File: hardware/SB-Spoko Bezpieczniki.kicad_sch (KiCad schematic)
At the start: 20 parts, among them IC1 STM32L4P5RET6, SW1 RESET, Y1 Crystal_GND24_Small

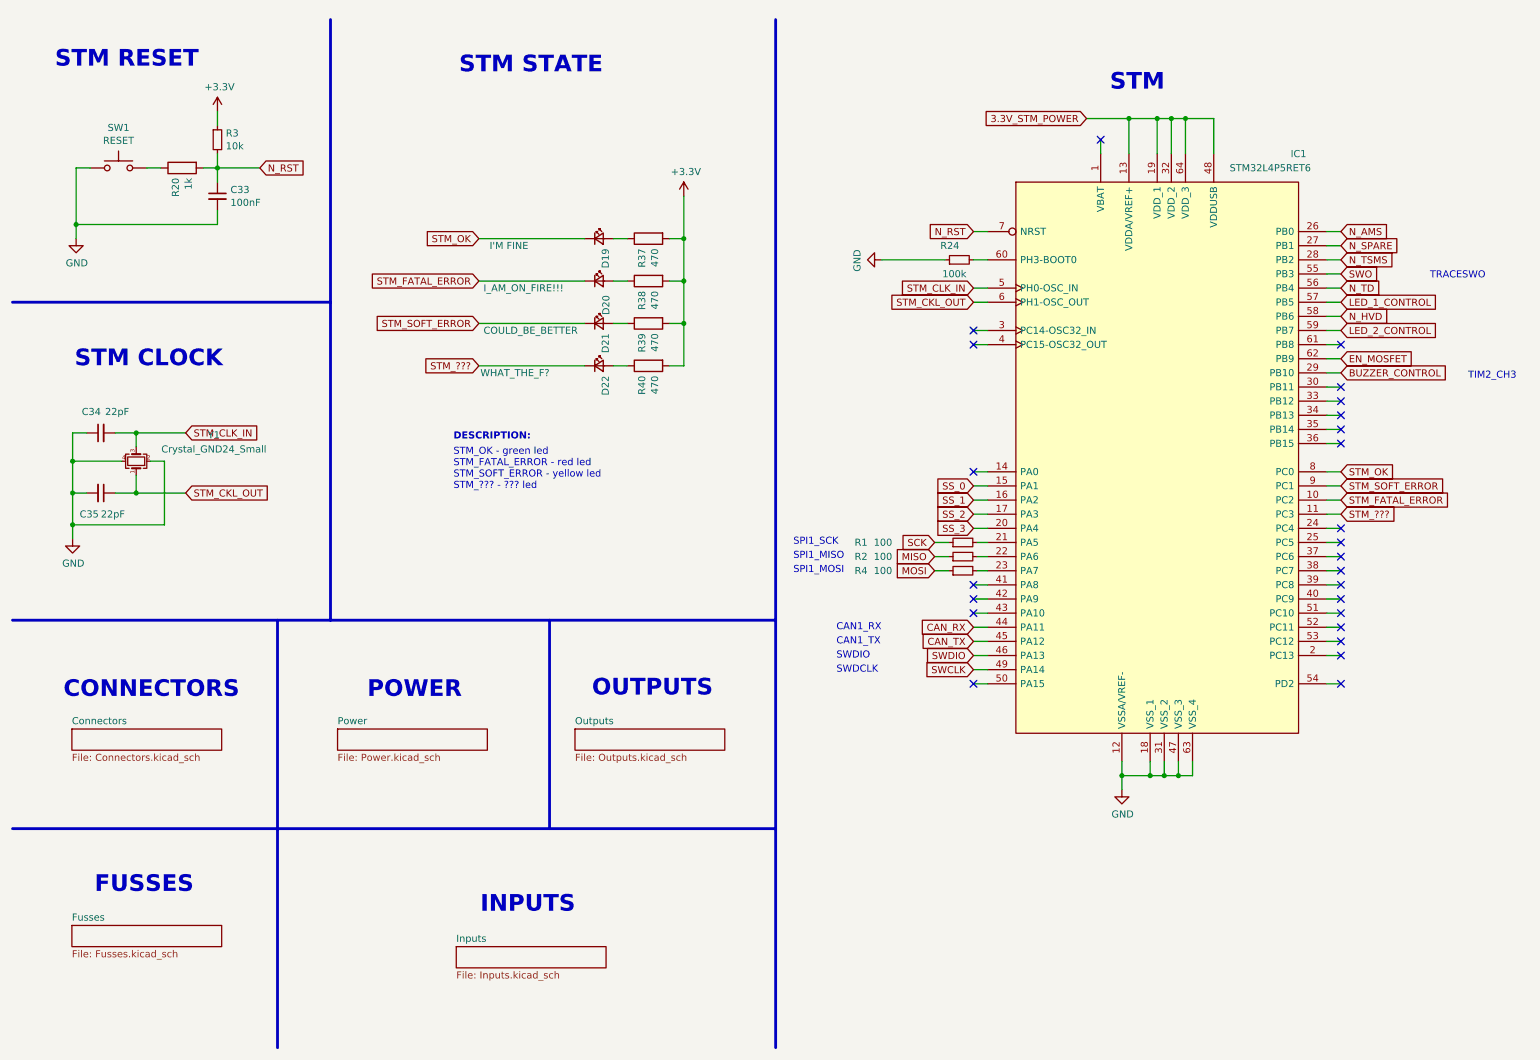
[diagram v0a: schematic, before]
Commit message: changed some footprints for clarity, and made some progress on board
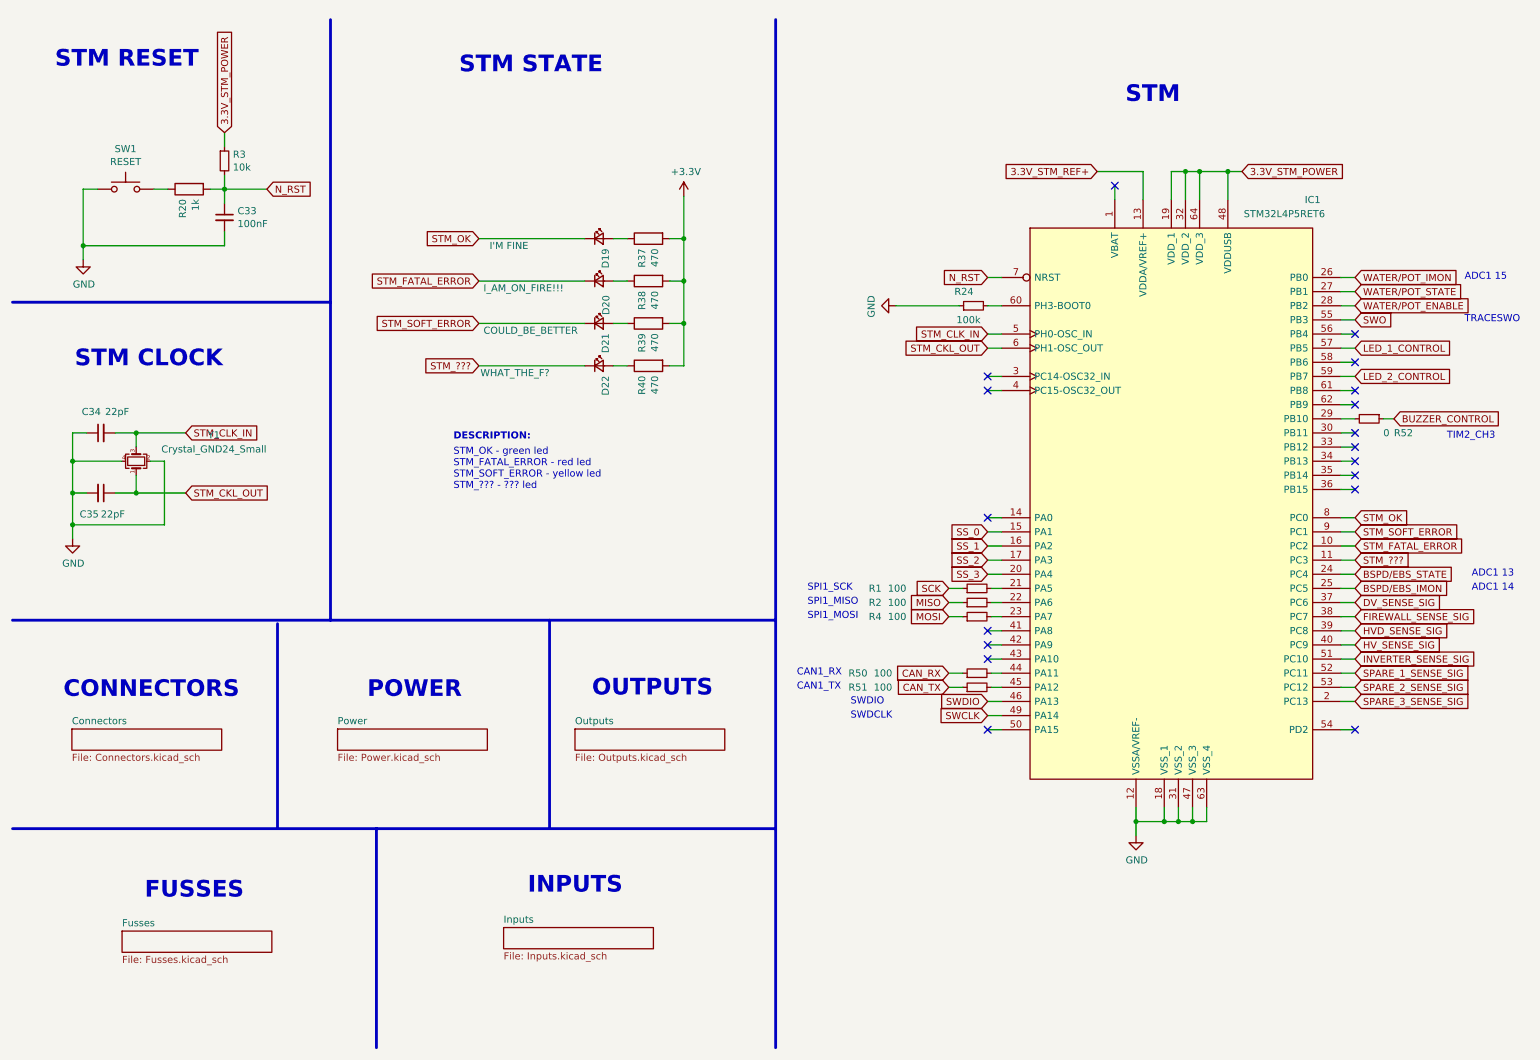
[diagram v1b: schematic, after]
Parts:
- added R50, R51: 100, Resistor_SMD:R_0603_1608Metric, symbol Device:R_Small
- added R52: 0, Resistor_SMD:R_0603_1608Metric, symbol Device:R_Small
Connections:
- net +3V3: no longer R3.1
- net 3.3V_STM_POWER: now also R3.1; no longer IC1.13 (VDDA/VREF+)
- net BUZZER_CONTROL: now also R52.1; no longer IC1.29 (PB10)
- net CAN_RX: now also R50.1; no longer IC1.44 (PA11)
- net CAN_TX: now also R51.1; no longer IC1.45 (PA12)
- net SPARE_3_SENSE_SIG: now reaches IC1.2 (PC13)
- net BSPD/EBS_STATE: now reaches IC1.24 (PC4)
- net BSPD/EBS_IMON: now reaches IC1.25 (PC5)
- net DV_SENSE_SIG: now reaches IC1.37 (PC6)
- net FIREWALL_SENSE_SIG: now reaches IC1.38 (PC7)
- net HVD_SENSE_SIG: now reaches IC1.39 (PC8)
- net HV_SENSE_SIG: now reaches IC1.40 (PC9)
- net INVERTER_SENSE_SIG: now reaches IC1.51 (PC10)
- net SPARE_1_SENSE_SIG: now reaches IC1.52 (PC11)
- net SPARE_2_SENSE_SIG: now reaches IC1.53 (PC12)
- net EN_MOSFET: no longer names the net of IC1.62 (PB9)
- net N_AMS renamed WATER/POT_IMON
- net N_HVD: no longer names the net of IC1.58 (PB6)
- net N_SPARE renamed WATER/POT_STATE
- net N_TD: no longer names the net of IC1.56 (PB4)
- net N_TSMS renamed WATER/POT_ENABLE
- new net: IC1.29 (PB10), R52.2
- new net: IC1.44 (PA11), R50.2
- new net: IC1.45 (PA12), R51.2
- new net 3.3V_STM_REF+: IC1.13 (VDDA/VREF+)
- no-connect marks 25 -> 18
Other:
- note added: "ADC1 13"
- note added: "ADC1 14"
- note added: "ADC1 15"
- moved on the sheet: C33, IC1, R1, R2, R20, R24, R3, R4, SW1
